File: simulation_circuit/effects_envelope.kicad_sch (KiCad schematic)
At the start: 13 parts, among them Q2 BC547B

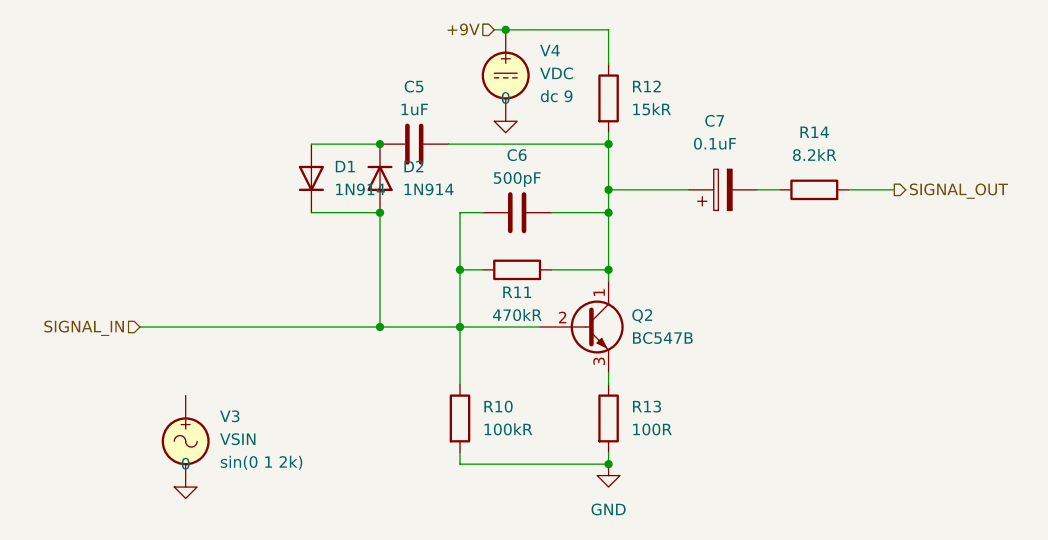
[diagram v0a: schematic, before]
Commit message: WIP
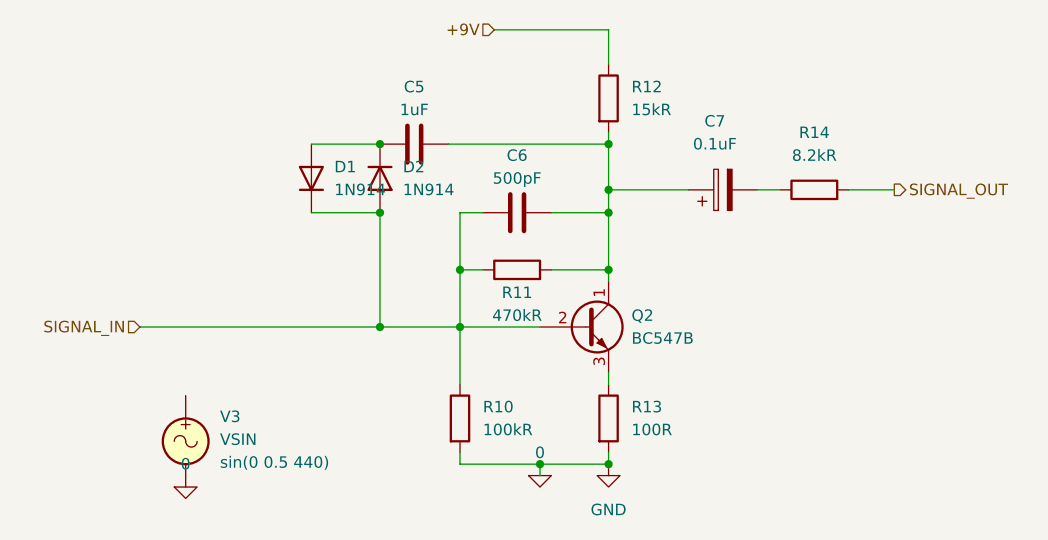
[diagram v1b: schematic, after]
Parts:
- removed V4: VDC, symbol Simulation_SPICE:VDC
- V3: Spice_Model sin(0 1 2k) -> sin(0 0.5 440)
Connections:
- net GND is gone; now on net 0: R10.2, R13.2
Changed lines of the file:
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@@
   (junction (at 154.94 95.25) (diameter 0) (color 0 0 0 0)
   )
+  (junction (at 147.32 116.84) (diameter 0) (color 0 0 0 0)
+  )
   (junction (at 129.54 88.9) (diameter 0) (color 0 0 0 0)
   )
@@
   (junction (at 154.94 86.36) (diameter 0) (color 0 0 0 0)
   )
-  (junction (at 143.51 68.58) (diameter 0) (color 0 0 0 0)
-  )
   (junction (at 154.94 81.28) (diameter 0) (color 0 0 0 0)
   )
@@
     (stroke (width 0) (type default) (color 0 0 0 0))
   )
-  (wire (pts (xy 143.51 68.58) (xy 154.94 68.58))
+  (wire (pts (xy 142.24 68.58) (xy 154.94 68.58))
     (stroke (width 0) (type default) (color 0 0 0 0))
   )
@@
     (stroke (width 0) (type default) (color 0 0 0 0))
   )
+  (wire (pts (xy 147.32 116.84) (xy 154.94 116.84))
+    (stroke (width 0) (type default) (color 0 0 0 0))
+  )
   (wire (pts (xy 154.94 106.68) (xy 154.94 107.95))
     (stroke (width 0) (type default) (color 0 0 0 0))
   )
+  (wire (pts (xy 102.87 101.6) (xy 129.54 101.6))
+    (stroke (width 0) (type default) (color 0 0 0 0))
+  )
   (wire (pts (xy 154.94 72.39) (xy 154.94 68.58))
     (stroke (width 0) (type default) (color 0 0 0 0))
@@
     (stroke (width 0) (type default) (color 0 0 0 0))
   )
-  (wire (pts (xy 102.87 101.6) (xy 129.54 101.6))
+  (wire (pts (xy 147.32 116.84) (xy 147.32 118.11))
     (stroke (width 0) (type default) (color 0 0 0 0))
   )
@@
     (stroke (width 0) (type default) (color 0 0 0 0))
   )
-  (wire (pts (xy 138.43 116.84) (xy 154.94 116.84))
+  (wire (pts (xy 138.43 116.84) (xy 147.32 116.84))
     (stroke (width 0) (type default) (color 0 0 0 0))
   )
@@
   )
   (wire (pts (xy 154.94 86.36) (xy 154.94 88.9))
-    (stroke (width 0) (type default) (color 0 0 0 0))
-  )
-  (wire (pts (xy 142.24 68.58) (xy 143.51 68.58))
     (stroke (width 0) (type default) (color 0 0 0 0))
   )
@@
   (symbol (lib_id "power:GND") (at 154.94 116.84 0) (unit 1)
     (in_bom yes) (on_board yes) (fields_autoplaced)
-    (property "Reference" "#PWR?" (id 0) (at 154.94 123.19 0)
+    (property "Reference" "#PWR0101" (id 0) (at 154.94 123.19 0)
       (effects (font (size 1.27 1.27)) hide)
     )
@@
   (symbol (lib_id "pspice:0") (at 107.95 119.38 0) (unit 1)
     (in_bom yes) (on_board yes) (fields_autoplaced)
-    (property "Reference" "#GND?" (id 0) (at 107.95 121.92 0)
+    (property "Reference" "#GND0101" (id 0) (at 107.95 121.92 0)
       (effects (font (size 1.27 1.27)) hide)
     )
@@
     (pin "2")
   )
-  (symbol (lib_id "pspice:0") (at 143.51 78.74 0) (unit 1)
-    (in_bom yes) (on_board yes) (fields_autoplaced)
-    (property "Reference" "#GND?" (id 0) (at 143.51 81.28 0)
-      (effects (font (size 1.27 1.27)) hide)
-    )
-    (property "Value" "0" (id 1) (at 143.51 76.2 0))
-    (property "Footprint" "" (id 2) (at 143.51 78.74 0)
-      (effects (font (size 1.27 1.27)) hide)
-    )
-    (property "Datasheet" "~" (id 3) (at 143.51 78.74 0)
+  (symbol (lib_id "pspice:0") (at 147.32 118.11 0) (unit 1)
+    (in_bom yes) (on_board yes) (fields_autoplaced)
+    (property "Reference" "#GND0102" (id 0) (at 147.32 120.65 0)
+      (effects (font (size 1.27 1.27)) hide)
+    )
+    (property "Value" "0" (id 1) (at 147.32 115.57 0))
+    (property "Footprint" "" (id 2) (at 147.32 118.11 0)
+      (effects (font (size 1.27 1.27)) hide)
+    )
+    (property "Datasheet" "~" (id 3) (at 147.32 118.11 0)
       (effects (font (size 1.27 1.27)) hide)
     )
@@
     (pin "2")
   )
-  (symbol (lib_id "Simulation_SPICE:VDC") (at 143.51 73.66 0) (unit 1)
-    (in_bom yes) (on_board yes) (fields_autoplaced)
-    (property "Reference" "V4" (id 0) (at 147.32 70.9301 0)
-      (effects (font (size 1.27 1.27)) (justify left))
-    )
-    (property "Value" "VDC" (id 1) (at 147.32 73.4701 0)
-      (effects (font (size 1.27 1.27)) (justify left))
-    )
-    (property "Footprint" "" (id 2) (at 143.51 73.66 0)
-      (effects (font (size 1.27 1.27)) hide)
-    )
-    (property "Datasheet" "~" (id 3) (at 143.51 73.66 0)
-      (effects (font (size 1.27 1.27)) hide)
-    )
-    (property "Spice_Netlist_Enabled" "Y" (id 4) (at 143.51 73.66 0)
-      (effects (font (size 1.27 1.27)) (justify left) hide)
-    )
-    (property "Spice_Primitive" "V" (id 5) (at 143.51 73.66 0)
-      (effects (font (size 1.27 1.27)) (justify left) hide)
-    )
-    (property "Spice_Model" "dc 9" (id 6) (at 147.32 76.0101 0)
-      (effects (font (size 1.27 1.27)) (justify left))
-    )
-    (pin "1")
-    (pin "2")
-  )
   (symbol (lib_id "Device:C_Polarized") (at 167.64 86.36 90) (unit 1)
     (in_bom yes) (on_board yes) (fields_autoplaced)
@@
       (effects (font (size 1.27 1.27)) (justify left) hide)
     )
-    (property "Spice_Model" "sin(0 1 2k)" (id 6) (at 111.76 116.6501 0)
-      (effects (font (size 1.27 1.27)) (justify left))
-    )
+    (property "Spice_Model" "sin(0 0.5 440)" (id 6) (at 111.76 116.6501 0)
+      (effects (font (size 1.27 1.27)) (justify left))
+    )
